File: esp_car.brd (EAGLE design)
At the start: 81.6 x 84 mm, 50 parts, among them IC1 TB6612FNG, IC2 LT1963ES8-3.3, SW2 SK-12D01, U2 ESP-WROOM-32_NOFLASH

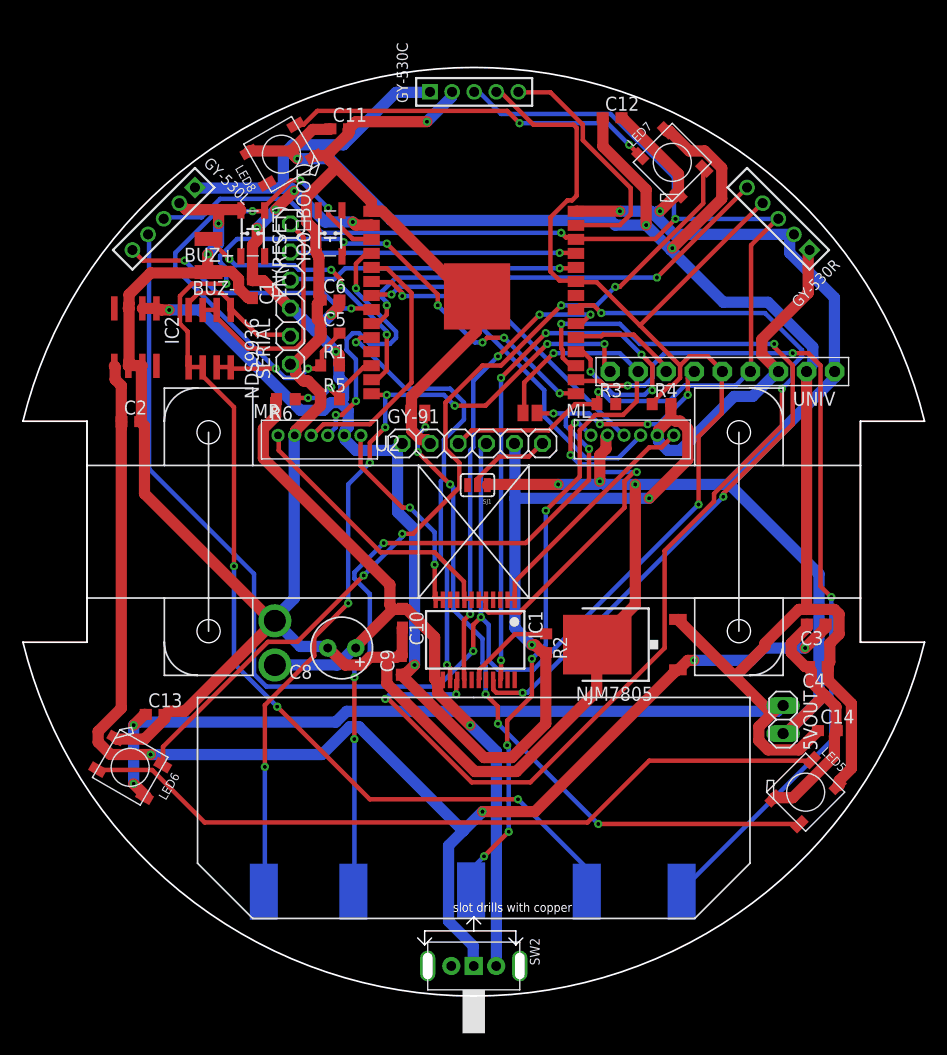
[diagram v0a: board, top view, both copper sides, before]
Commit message: daily
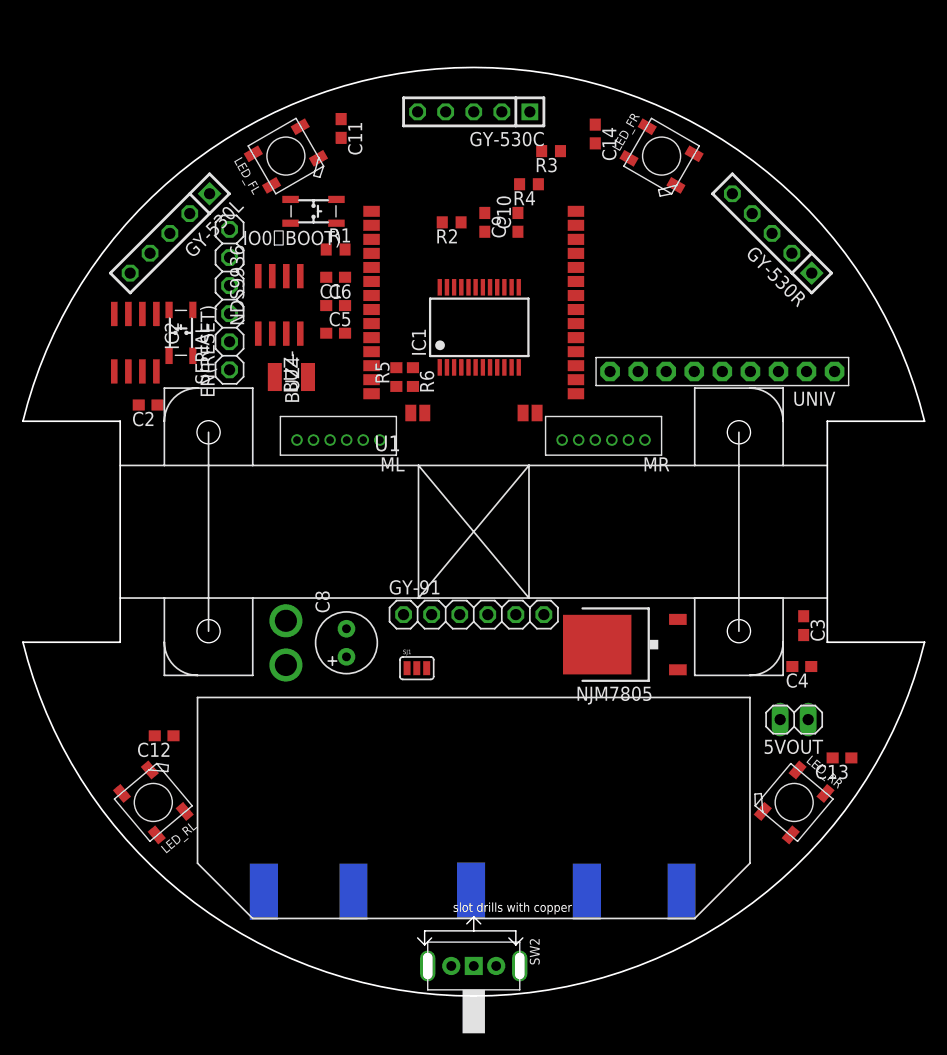
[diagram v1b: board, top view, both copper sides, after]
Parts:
- removed LED5, LED6, LED7, LED8: WS2812B5050, adafruit:WS2812B
- added LED_FL, LED_FR, LED_RL, LED_RR: WS2812B5050, adafruit:WS2812B
- GY-530C, GY-530L, GY-530R: device pinhead:1X05M -> pinhead:1X05
- moved C12 69.1 mm to (12.0, 21.5), turned to 180 degrees
- moved C13 62.3 mm to (73.3, 19.5), turned to 180 degrees
- moved C14 57.9 mm to (51.0, 76.0), turned to 270 degrees
- moved C9 40.8 mm to (41.0, 68.0), turned to 270 degrees
- moved R2 39.0 mm to (38.0, 68.0), turned to 180 degrees
- moved C10 37.3 mm to (44.0, 68.0), turned to 90 degrees
- moved MR 36.3 mm to (57.0, 47.0), turned to 180 degrees
- moved IC1 28.3 mm to (40.5, 58.5), turned to 0 degrees
- moved R3 23.4 mm to (47.0, 74.5), turned to 180 degrees
- moved R4 23.2 mm to (45.0, 71.5), turned to 180 degrees
- moved SJ1 17.5 mm to (34.9, 27.6), turned to 0 degrees
- moved ML 16.4 mm to (33.0, 47.0), turned to 180 degrees
- moved GY-91 15.5 mm to (40.0, 32.5)
- moved BUZ+ 15.4 mm to (25.0, 54.0), turned to 0 degrees
- moved R6 11.7 mm to (34.5, 54.0), turned to 270 degrees
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- renumbered U2 to U1
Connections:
- net N$10 renamed ML+
- net N$11 renamed ML-
- net N$12 renamed MR-
- net N$13 renamed MR+
- removed net N$2: IC2.8
- net +3V3: now also R3.2
- net +5V: now also LED_FL.1-VDD, LED_FR.1-VDD, LED_RL.1-VDD, LED_RR.1-VDD; no longer LED5.1-VDD, LED6.1-VDD, LED7.1-VDD, LED8.1-VDD
- net GND: now also LED_FL.3-GND, LED_FR.3-GND, LED_RL.3-GND, LED_RR.3-GND; no longer LED5.3-GND, LED6.3-GND, LED7.3-GND, LED8.3-GND, U1.GND
- net N$15: now also LED_FR.4-DIN, LED_RR.2-DOUT; no longer LED7.2-DOUT, LED8.4-DIN
- net N$18: now also LED_FL.4-DIN; no longer LED5.4-DIN
- net N$19: now also GY-530L.5; no longer GY-530R.5
- net N$3: now also GY-530C.5; no longer GY-530L.5
- net N$5: now also GY-530R.5; no longer GY-530C.5
- net N$6: now also LED_FL.2-DOUT, LED_RL.4-DIN; no longer LED5.2-DOUT, LED6.4-DIN
- net N$9: now also LED_RL.2-DOUT, LED_RR.4-DIN; no longer LED6.2-DOUT, LED7.4-DIN
- net VCC: now also IC2.8
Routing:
- net GND: track 385.3 -> 0.00 mm, vias 8 -> 0
- net +5V: track 235.3 -> 0.00 mm, vias 5 -> 0
- net +3V3: track 217.0 -> 0.00 mm, vias 10 -> 0
- net I2C_SDA: track 190.6 -> 0.00 mm, vias 3 -> 0
- net I2C_SCL: track 129.1 -> 0.00 mm, vias 3 -> 0
- net VCC: track 128.0 -> 0.00 mm, vias 4 -> 0
- net IO0: track 126.0 -> 0.00 mm, vias 10 -> 0
- net MR_IN2: track 95.8 -> 0.00 mm, vias 4 -> 0
- net N$9: track 80.6 -> 0.00 mm, vias 4 -> 0
- net IO2: track 79.2 -> 0.00 mm, vias 8 -> 0
- net IO4: track 78.4 -> 0.00 mm, vias 3 -> 0
- net IO12: track 76.1 -> 0.00 mm, vias 8 -> 0
- net VDD: track 74.1 -> 0.00 mm, vias 1 -> 0
- net ML_IN1: track 70.9 -> 0.00 mm, vias 4 -> 0
- net IO15: track 69.8 -> 0.00 mm, vias 6 -> 0
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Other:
- outline, holes or cut-outs redrawn
